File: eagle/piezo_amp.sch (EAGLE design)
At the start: 3 parts, among them U1 TLC2262CP

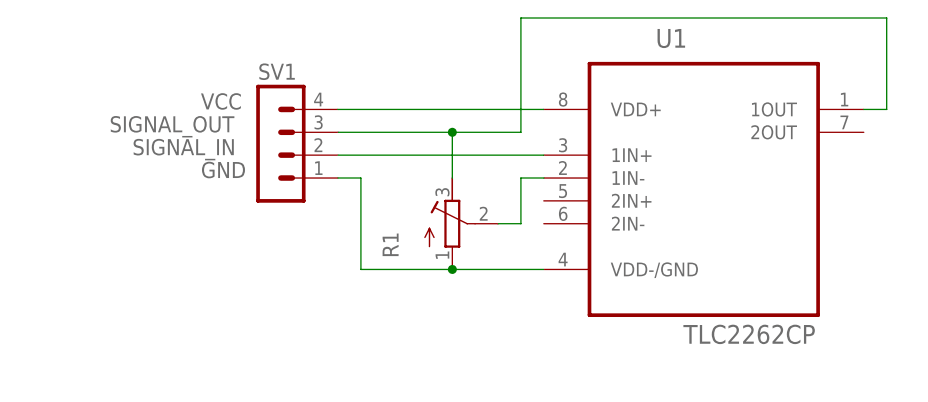
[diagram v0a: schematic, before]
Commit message: edit schematics
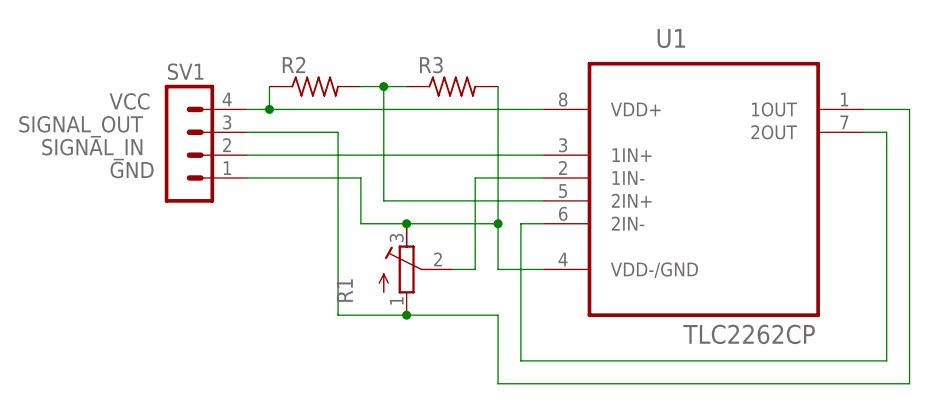
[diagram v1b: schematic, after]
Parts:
- added R2, R3: (no value), rcl:R-US_0204/5
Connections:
- new net N$1: U1.2IN-, U1.2OUT
- new net N$2: R2.2, R3.1, U1.2IN+
- net GND: now also R1.E, R3.2; no longer R1.A
- net SIGNAL_OUT: now also R1.A; no longer R1.E
- net VCC: now also R2.1
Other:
- moved on the sheet: R1, SV1
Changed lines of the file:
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@@
 <part name="SV1" library="con-lstb" deviceset="MA04-1" device=""/>
 <part name="R1" library="resistor" deviceset="R-TRIMM" device="3296W"/>
+<part name="R2" library="rcl" deviceset="R-US_" device="0204/5"/>
+<part name="R3" library="rcl" deviceset="R-US_" device="0204/5"/>
 </parts>
 <sheets>
@@
 <instance part="FRAME1" gate="G$1" x="5.08" y="22.86"/>
 <instance part="FRAME1" gate="G$2" x="152.4" y="22.86"/>
-<instance part="SV1" gate="1" x="83.82" y="134.62"/>
-<instance part="R1" gate="G$1" x="104.14" y="124.46"/>
+<instance part="SV1" gate="1" x="73.66" y="134.62"/>
+<instance part="R1" gate="G$1" x="99.06" y="119.38"/>
+<instance part="R2" gate="G$1" x="88.9" y="139.7"/>
+<instance part="R3" gate="G$1" x="104.14" y="139.7"/>
 </instances>
 <busses>
@@
 <pinref part="SV1" gate="1" pin="4"/>
 <pinref part="U1" gate="A" pin="VDD+"/>
-<wire x1="91.44" y1="137.16" x2="114.3" y2="137.16" width="0.1524" layer="91"/>
-<label x="76.2" y="137.16" size="1.778" layer="95"/>
+<wire x1="81.28" y1="137.16" x2="83.82" y2="137.16" width="0.1524" layer="91"/>
+<label x="66.04" y="137.16" size="1.778" layer="95"/>
+<pinref part="R2" gate="G$1" pin="1"/>
+<wire x1="83.82" y1="137.16" x2="114.3" y2="137.16" width="0.1524" layer="91"/>
+<wire x1="83.82" y1="139.7" x2="83.82" y2="137.16" width="0.1524" layer="91"/>
+<junction x="83.82" y="137.16"/>
 </segment>
 </net>
@@
 <pinref part="SV1" gate="1" pin="2"/>
 <pinref part="U1" gate="A" pin="1IN+"/>
-<wire x1="91.44" y1="132.08" x2="114.3" y2="132.08" width="0.1524" layer="91"/>
-<label x="68.58" y="132.08" size="1.778" layer="95"/>
+<wire x1="81.28" y1="132.08" x2="114.3" y2="132.08" width="0.1524" layer="91"/>
+<label x="58.42" y="132.08" size="1.778" layer="95"/>
 </segment>
 </net>
 <net name="SIGNAL_OUT" class="0">
 <segment>
+<wire x1="154.94" y1="106.68" x2="154.94" y2="137.16" width="0.1524" layer="91"/>
+<pinref part="U1" gate="A" pin="1OUT"/>
+<wire x1="149.86" y1="137.16" x2="154.94" y2="137.16" width="0.1524" layer="91"/>
+<wire x1="109.22" y1="114.3" x2="109.22" y2="106.68" width="0.1524" layer="91"/>
+<wire x1="109.22" y1="106.68" x2="154.94" y2="106.68" width="0.1524" layer="91"/>
 <pinref part="SV1" gate="1" pin="3"/>
-<wire x1="91.44" y1="134.62" x2="104.14" y2="134.62" width="0.1524" layer="91"/>
-<wire x1="104.14" y1="134.62" x2="111.76" y2="134.62" width="0.1524" layer="91"/>
-<wire x1="111.76" y1="134.62" x2="111.76" y2="147.32" width="0.1524" layer="91"/>
-<wire x1="111.76" y1="147.32" x2="152.4" y2="147.32" width="0.1524" layer="91"/>
-<wire x1="152.4" y1="147.32" x2="152.4" y2="137.16" width="0.1524" layer="91"/>
-<pinref part="U1" gate="A" pin="1OUT"/>
-<wire x1="152.4" y1="137.16" x2="149.86" y2="137.16" width="0.1524" layer="91"/>
-<pinref part="R1" gate="G$1" pin="E"/>
-<wire x1="104.14" y1="129.54" x2="104.14" y2="134.62" width="0.1524" layer="91"/>
-<junction x="104.14" y="134.62"/>
-<label x="66.04" y="134.62" size="1.778" layer="95"/>
+<wire x1="81.28" y1="134.62" x2="91.44" y2="134.62" width="0.1524" layer="91"/>
+<wire x1="91.44" y1="134.62" x2="91.44" y2="114.3" width="0.1524" layer="91"/>
+<label x="55.88" y="134.62" size="1.778" layer="95"/>
+<pinref part="R1" gate="G$1" pin="A"/>
+<wire x1="91.44" y1="114.3" x2="99.06" y2="114.3" width="0.1524" layer="91"/>
+<wire x1="109.22" y1="114.3" x2="99.06" y2="114.3" width="0.1524" layer="91"/>
+<junction x="99.06" y="114.3"/>
 </segment>
 </net>
 <net name="GND" class="0">
 <segment>
+<pinref part="R3" gate="G$1" pin="2"/>
+<wire x1="109.22" y1="139.7" x2="109.22" y2="124.46" width="0.1524" layer="91"/>
+<pinref part="U1" gate="A" pin="VDD-/GND"/>
+<wire x1="109.22" y1="124.46" x2="109.22" y2="119.38" width="0.1524" layer="91"/>
+<wire x1="109.22" y1="119.38" x2="114.3" y2="119.38" width="0.1524" layer="91"/>
+<wire x1="93.98" y1="129.54" x2="93.98" y2="124.46" width="0.1524" layer="91"/>
 <pinref part="SV1" gate="1" pin="1"/>
-<wire x1="91.44" y1="129.54" x2="93.98" y2="129.54" width="0.1524" layer="91"/>
-<wire x1="93.98" y1="129.54" x2="93.98" y2="119.38" width="0.1524" layer="91"/>
-<pinref part="U1" gate="A" pin="VDD-/GND"/>
-<wire x1="93.98" y1="119.38" x2="104.14" y2="119.38" width="0.1524" layer="91"/>
-<pinref part="R1" gate="G$1" pin="A"/>
-<wire x1="104.14" y1="119.38" x2="114.3" y2="119.38" width="0.1524" layer="91"/>
-<junction x="104.14" y="119.38"/>
-<label x="76.2" y="129.54" size="1.778" layer="95"/>
+<wire x1="81.28" y1="129.54" x2="93.98" y2="129.54" width="0.1524" layer="91"/>
+<label x="66.04" y="129.54" size="1.778" layer="95"/>
+<pinref part="R1" gate="G$1" pin="E"/>
+<wire x1="93.98" y1="124.46" x2="99.06" y2="124.46" width="0.1524" layer="91"/>
+<wire x1="99.06" y1="124.46" x2="109.22" y2="124.46" width="0.1524" layer="91"/>
+<junction x="99.06" y="124.46"/>
+<junction x="109.22" y="124.46"/>
 </segment>
 </net>
 <net name="N$5" class="0">
 <segment>
+<pinref part="U1" gate="A" pin="1IN-"/>
+<wire x1="106.68" y1="129.54" x2="114.3" y2="129.54" width="0.1524" layer="91"/>
+<wire x1="106.68" y1="119.38" x2="106.68" y2="129.54" width="0.1524" layer="91"/>
 <pinref part="R1" gate="G$1" pin="S"/>
-<wire x1="109.22" y1="124.46" x2="111.76" y2="124.46" width="0.1524" layer="91"/>
-<wire x1="111.76" y1="124.46" x2="111.76" y2="129.54" width="0.1524" layer="91"/>
-<pinref part="U1" gate="A" pin="1IN-"/>
-<wire x1="111.76" y1="129.54" x2="114.3" y2="129.54" width="0.1524" layer="91"/>
+<wire x1="104.14" y1="119.38" x2="106.68" y2="119.38" width="0.1524" layer="91"/>
 </segment>
 </net>
+<net name="N$1" class="0">
+<segment>
+<pinref part="U1" gate="A" pin="2IN-"/>
+<wire x1="114.3" y1="124.46" x2="111.76" y2="124.46" width="0.1524" layer="91"/>
+<wire x1="111.76" y1="124.46" x2="111.76" y2="109.22" width="0.1524" layer="91"/>
+<wire x1="111.76" y1="109.22" x2="152.4" y2="109.22" width="0.1524" layer="91"/>
+<wire x1="152.4" y1="109.22" x2="152.4" y2="134.62" width="0.1524" layer="91"/>
+<pinref part="U1" gate="A" pin="2OUT"/>
+<wire x1="152.4" y1="134.62" x2="149.86" y2="134.62" width="0.1524" layer="91"/>
+</segment>
+</net>
+<net name="N$2" class="0">
+<segment>
+<pinref part="R2" gate="G$1" pin="2"/>
+<pinref part="R3" gate="G$1" pin="1"/>
+<wire x1="93.98" y1="139.7" x2="96.52" y2="139.7" width="0.1524" layer="91"/>
+<pinref part="U1" gate="A" pin="2IN+"/>
+<wire x1="96.52" y1="139.7" x2="99.06" y2="139.7" width="0.1524" layer="91"/>
+<wire x1="114.3" y1="127" x2="96.52" y2="127" width="0.1524" layer="91"/>
+<wire x1="96.52" y1="127" x2="96.52" y2="139.7" width="0.1524" layer="91"/>
+<junction x="96.52" y="139.7"/>
+</segment>
+</net>
